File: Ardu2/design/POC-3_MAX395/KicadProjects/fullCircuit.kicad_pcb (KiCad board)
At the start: 2 copper layers, 162.6 x 133.3 mm, 126 parts, among them P1 CONN_01X02, P7 CONN_01X15, U1 Pyboard, U10 MAX395, U11 MAX395, U12 MAX395, U13 MAX395, U14 MAX395, U15 MAX395, U16 MAX395, U17 MAX395, U18 MAX395, U2 LM2596, U3 LM2596, U4 Vactrol, U5 MAX395, U6 MAX395, U7 MAX395, U8 MAX395, U9 MAX395

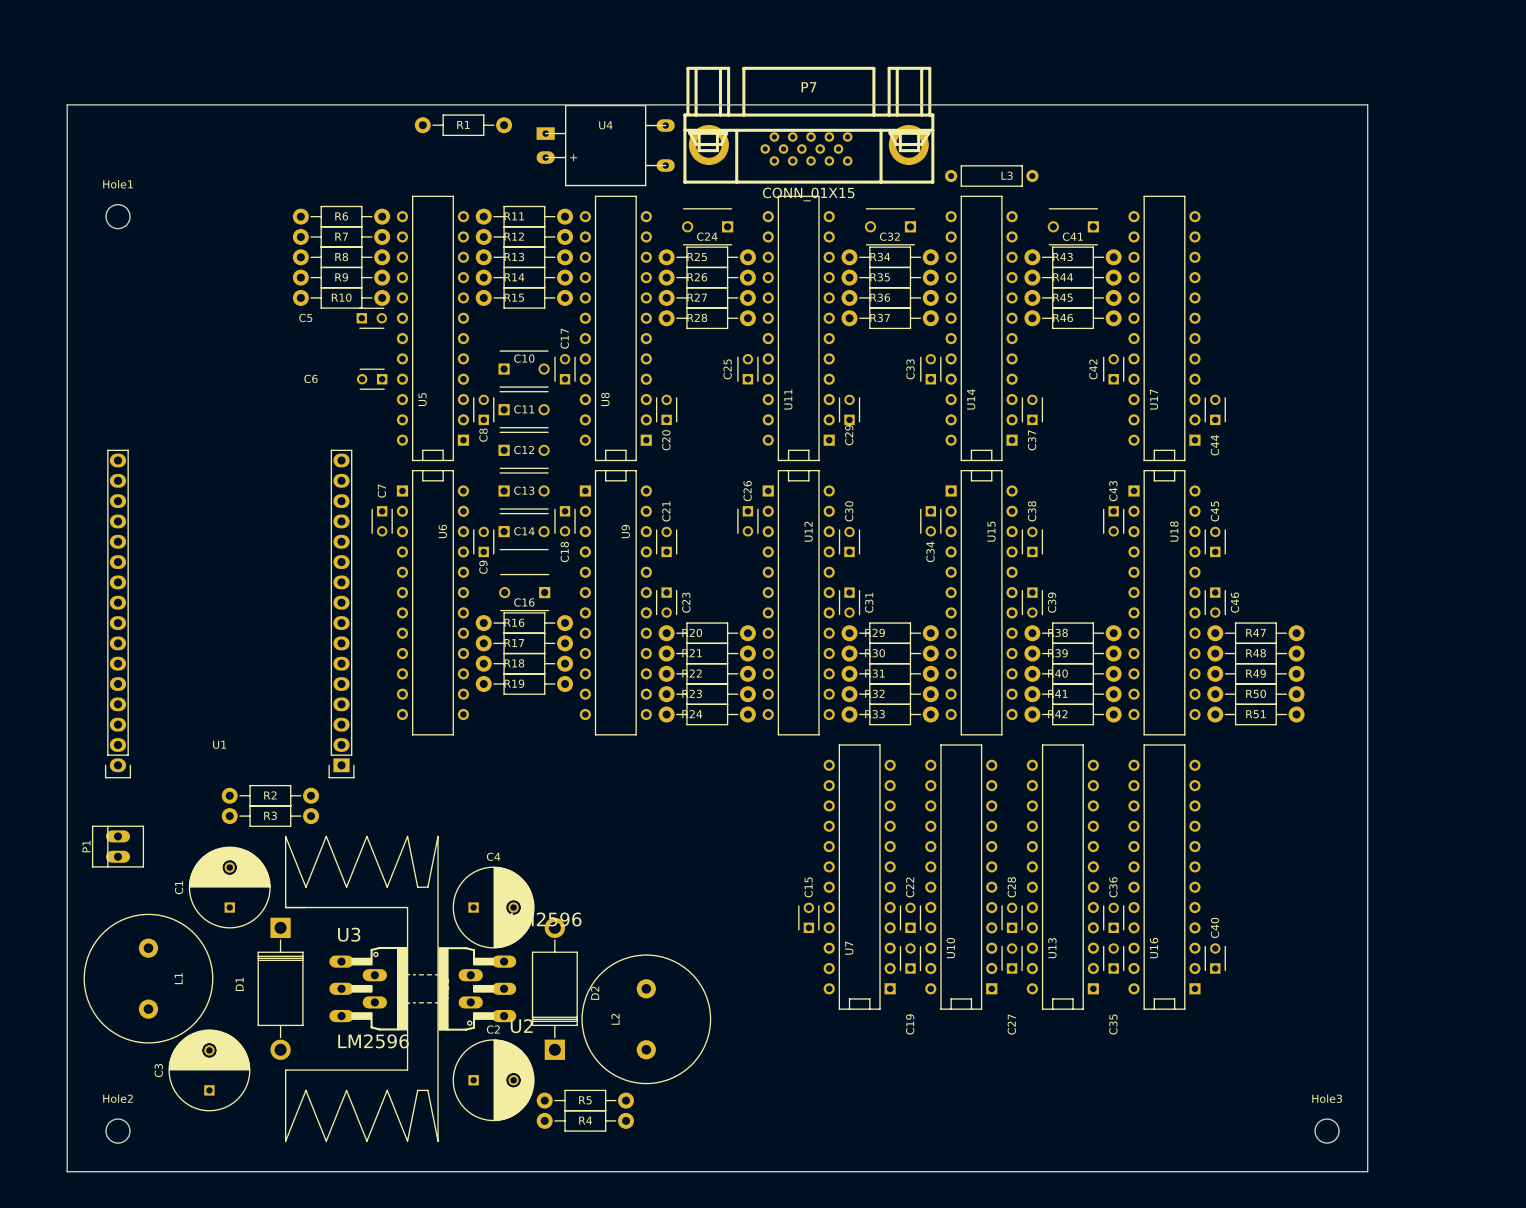
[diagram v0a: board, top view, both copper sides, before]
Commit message: another pcb version...
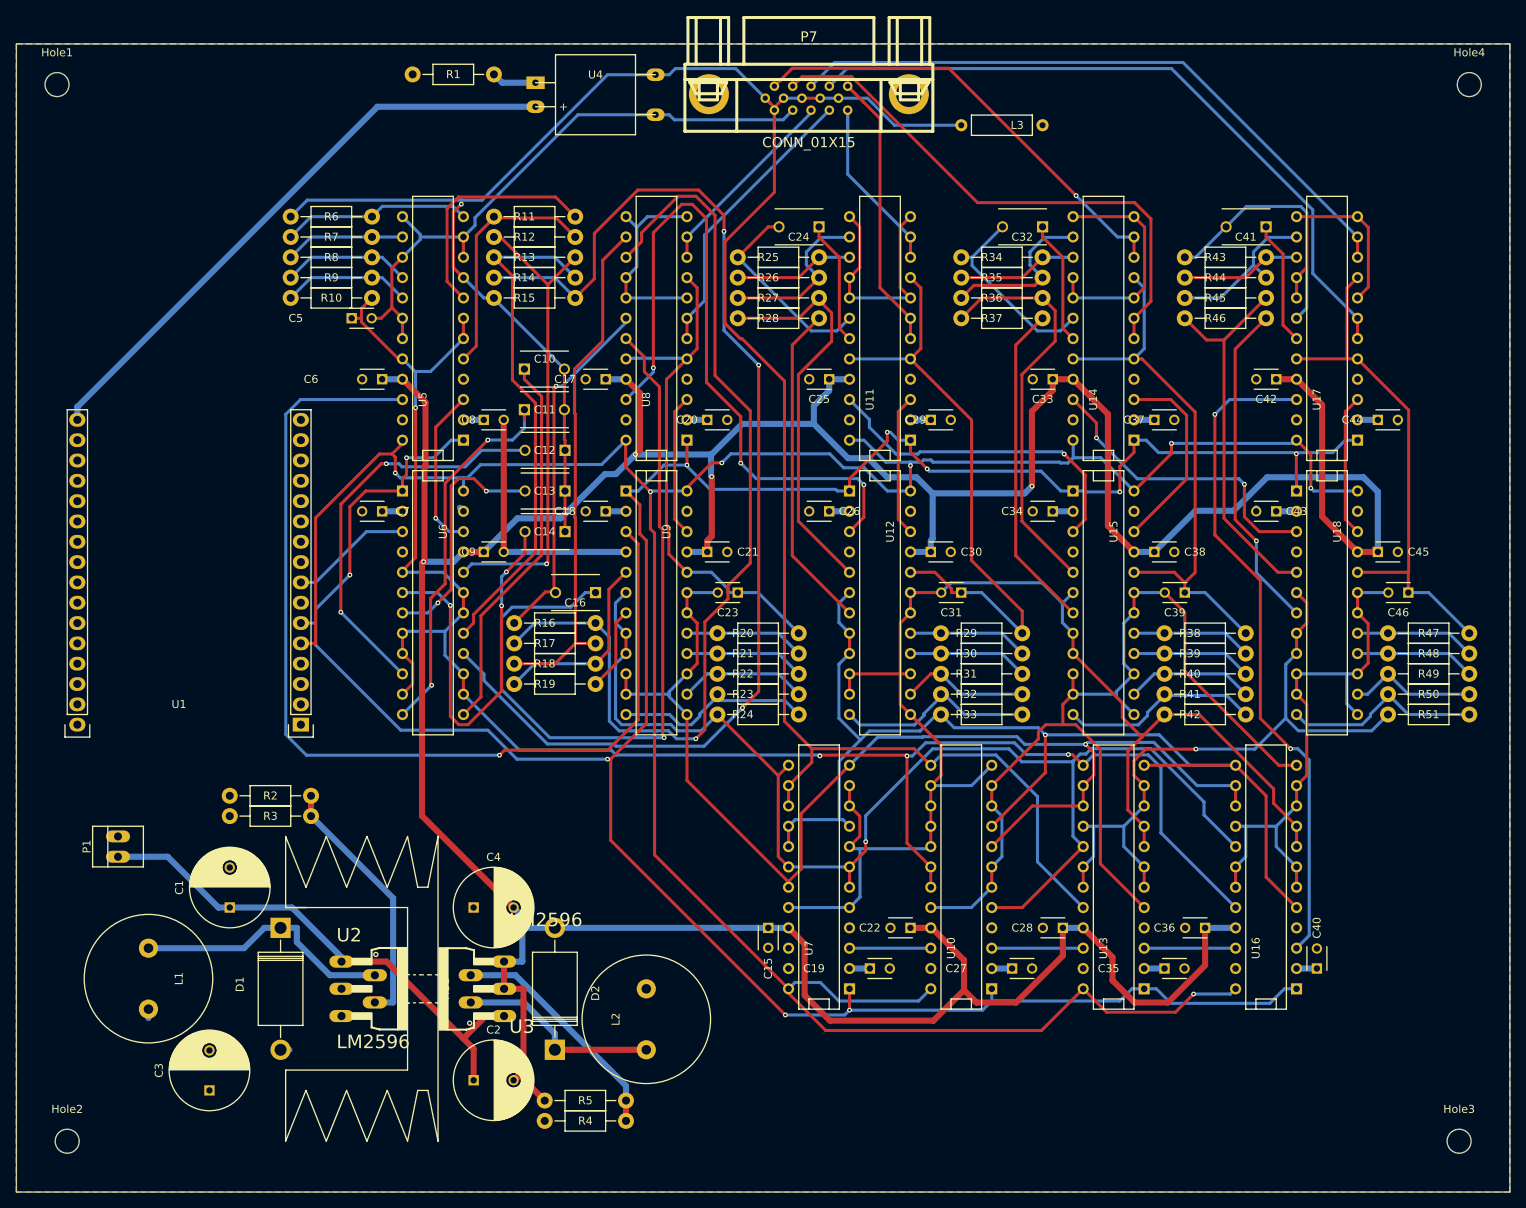
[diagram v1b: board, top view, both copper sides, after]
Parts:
- added Hole4: MountingHole_3mm, Mounting_Holes:MountingHole_3mm, F.Cu at (243.8, 22.9)
- moved C46 24.1 mm to (236.2, 86.4), turned to 180 degrees
- moved C41 21.6 mm to (218.4, 40.6)
- moved R47 21.6 mm to (238.8, 91.4)
- moved R48 21.6 mm to (238.8, 94.0)
- moved R49 21.6 mm to (238.8, 96.5)
- moved R50 21.6 mm to (238.8, 99.1)
- moved R51 21.6 mm to (238.8, 101.6)
- moved C42 20.3 mm to (219.7, 59.7), turned to 180 degrees
- moved C43 20.3 mm to (219.7, 76.2), turned to 180 degrees
- moved C44 20.3 mm to (232.4, 64.8), turned to 0 degrees
- moved C45 20.3 mm to (232.4, 81.3), turned to 0 degrees
- moved U17 20.3 mm to (226.1, 53.3)
- moved U18 20.3 mm to (226.1, 87.6)
- moved C39 19.1 mm to (208.3, 86.4), turned to 180 degrees
- moved R43 19.1 mm to (213.4, 44.5)
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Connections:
- L3 pad 2: Net-(L3-Pad2) -> /MIn-
- P7 pad 10: Net-(L3-Pad2) -> /MIn-
- P7 pad 6: Net-(L3-Pad2) -> /MIn-
- P7 pad 7: Net-(L3-Pad2) -> /MIn-
- P7 pad 8: Net-(L3-Pad2) -> /MIn-
- P7 pad 9: Net-(L3-Pad2) -> /MIn-
- U1 pad 1: /ShuntControl -> (no net)
- U1 pad 17: (no net) -> /ShuntControl
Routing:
- net /V-: track 0.00 -> 484.7 mm, vias 0 -> 4
- net /CLK: track 0.00 -> 349.3 mm, vias 0 -> 10
- net /CS: track 0.00 -> 345.4 mm, vias 0 -> 7
- net /MIn-: track 0.00 -> 293.2 mm, vias 0 -> 1
- net /MIn+: track 0.00 -> 220.0 mm, vias 0 -> 4
- net /BOut-: track 0.00 -> 176.8 mm
- net /DOut-: track 0.00 -> 156.4 mm, vias 0 -> 1
- net /DOut+: track 0.00 -> 151.7 mm, vias 0 -> 1
- net Net-(R14-Pad1): track 0.00 -> 146.4 mm, vias 0 -> 3
- net /COut-: track 0.00 -> 140.5 mm, vias 0 -> 1
- net /BOut+: track 0.00 -> 127.0 mm
- net Net-(U5-Pad22): track 0.00 -> 126.5 mm, vias 0 -> 1
- net Net-(R16-Pad2): track 0.00 -> 121.9 mm, vias 0 -> 1
- net Net-(C16-Pad1): track 0.00 -> 96.7 mm, vias 0 -> 1
- net /A+: track 0.00 -> 87.1 mm
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- added copper zone on B.Cu, net /V+
- added copper zone on F.Cu, net GND
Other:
- board size 162.6 x 133.3 mm -> 186.7 x 143.5 mm
